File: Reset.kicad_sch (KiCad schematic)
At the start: 5 parts, among them U6 74LVC1G04

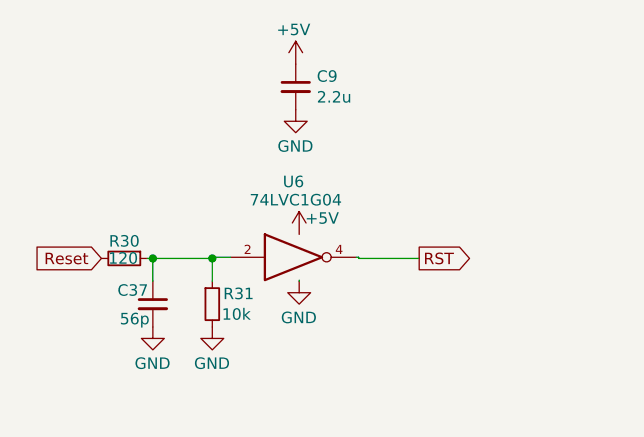
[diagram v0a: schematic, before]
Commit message: VER2.0 Отправил в резонит
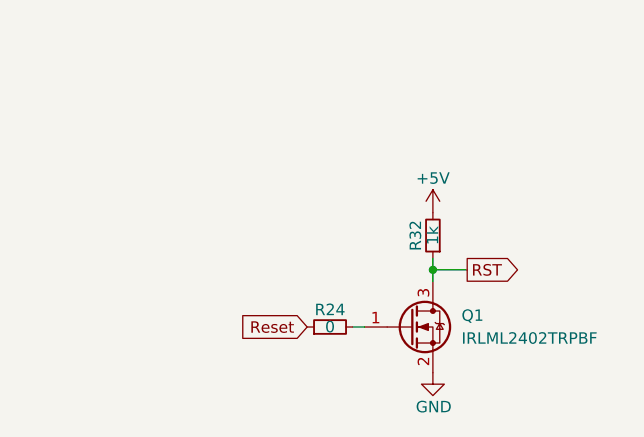
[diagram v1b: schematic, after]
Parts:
- removed C37: 56p, Capacitor_SMD:C_0805_2012Metric_Pad1.18x1.45mm_HandSolder, symbol Device:C_Small
- removed C9: 2.2u, Capacitor_SMD:C_0805_2012Metric_Pad1.18x1.45mm_HandSolder, symbol Device:C_Small
- removed R30: 120, Resistor_SMD:R_0805_2012Metric_Pad1.20x1.40mm_HandSolder, symbol Device:R_Small
- removed R31: 10k, Resistor_SMD:R_0805_2012Metric_Pad1.20x1.40mm_HandSolder, symbol Device:R_Small
- removed U6: 74LVC1G04, Package_TO_SOT_SMD:SOT-23-5_HandSoldering, symbol 74xGxx:74LVC1G04
- added Q1: IRLML2402TRPBF, Package_TO_SOT_SMD:SOT-23, symbol Transistor_FET:2N7002
- added R24: 0, Resistor_SMD:R_0805_2012Metric_Pad1.20x1.40mm_HandSolder, symbol Device:R_Small
- added R32: 1k, Resistor_SMD:R_0805_2012Metric_Pad1.20x1.40mm_HandSolder, symbol Device:R_Small
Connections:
- net +5V: now also R32.2
- net GND: now also Q1.2 (S)
- net RST: now also Q1.3 (D), R32.1
- net Reset: now also R24.1
- new net: Q1.1 (G), R24.2
